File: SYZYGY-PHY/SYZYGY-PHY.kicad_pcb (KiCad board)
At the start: 4 copper layers, 57.7 x 28 mm, 36 parts, among them J1 QTH-020-01-X-D-DP-A, J2 ARJM11C7-502-KB-EW2, J3 Conn_01x08, U1 GPY111, Y1 Crystal_GND24

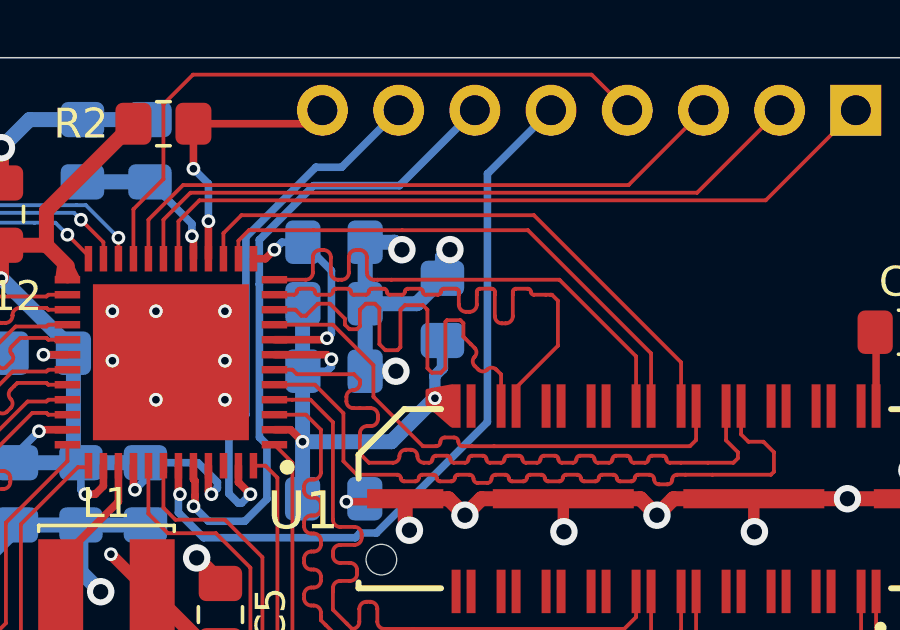
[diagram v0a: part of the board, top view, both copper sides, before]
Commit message: more length tuning
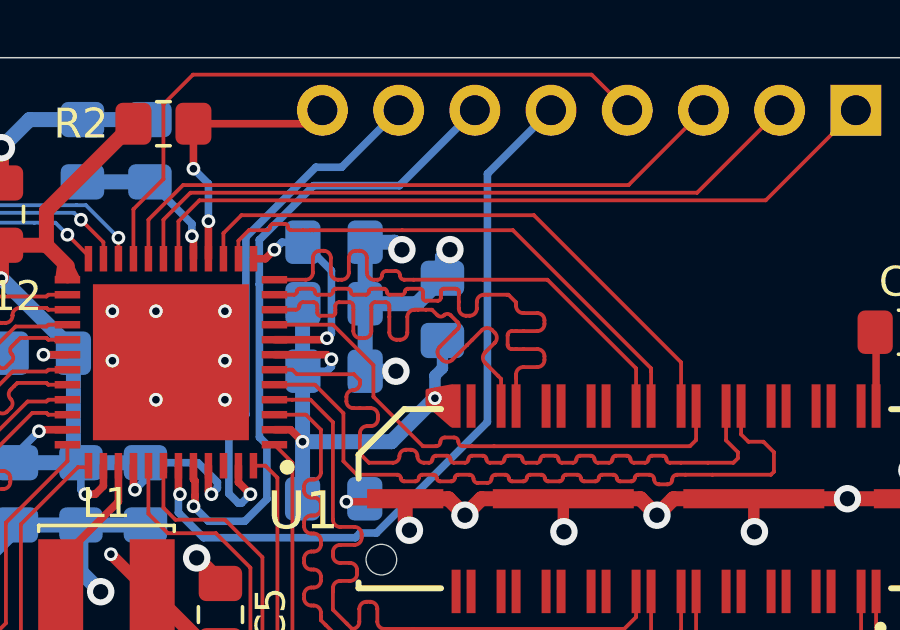
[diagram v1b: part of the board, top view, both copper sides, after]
